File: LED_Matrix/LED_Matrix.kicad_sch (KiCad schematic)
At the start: 21 parts, among them J1 Conn_01x02, U1 NE555P

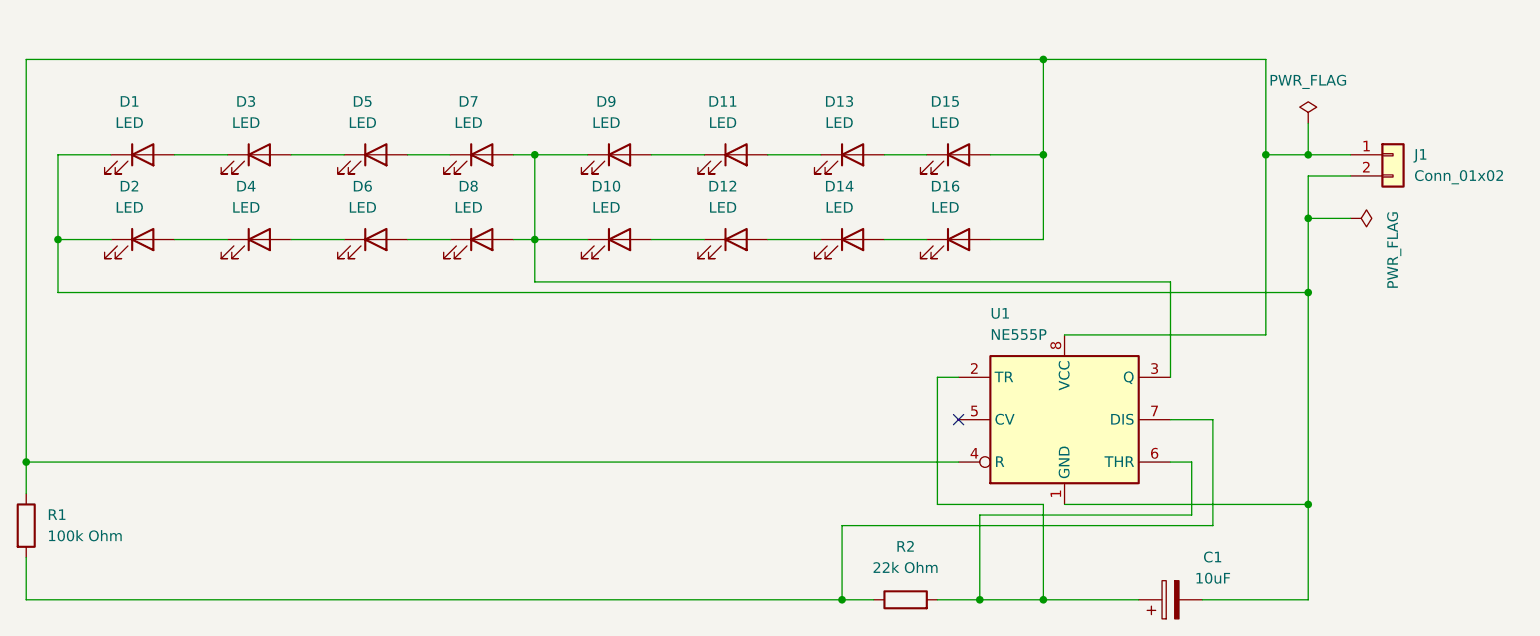
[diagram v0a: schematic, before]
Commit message: 20230812_1329
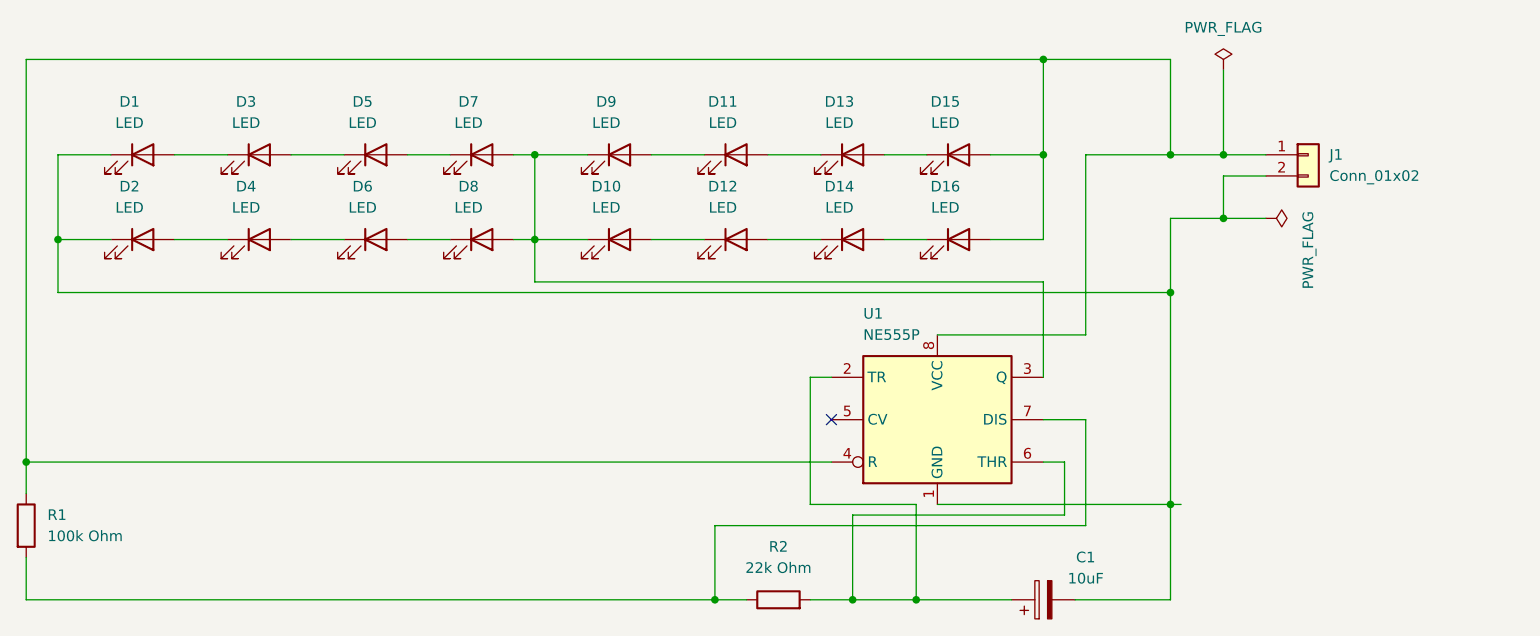
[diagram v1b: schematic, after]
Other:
- company: (none) -> DOSTI. Resource Center
- title: (none) -> LED_Matrix
- moved on the sheet: C1, J1, R2, U1
